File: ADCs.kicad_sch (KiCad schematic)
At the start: 25 parts, among them J10 Conn_01x03, J11 Conn_01x03, J12 Conn_01x03, J13 Conn_01x03, J14 Conn_01x03, J15 Conn_01x03, J16 Conn_01x03, J17 Conn_01x03, J2 Conn_01x03, J3 Conn_01x03, J4 Conn_01x03, J5 Conn_01x03, J6 Conn_01x03, J7 Conn_01x03, J8 Conn_01x03, J9 Conn_01x03, U13 TCA9517ADGK, U3 ADS7828, U4 ADS7828

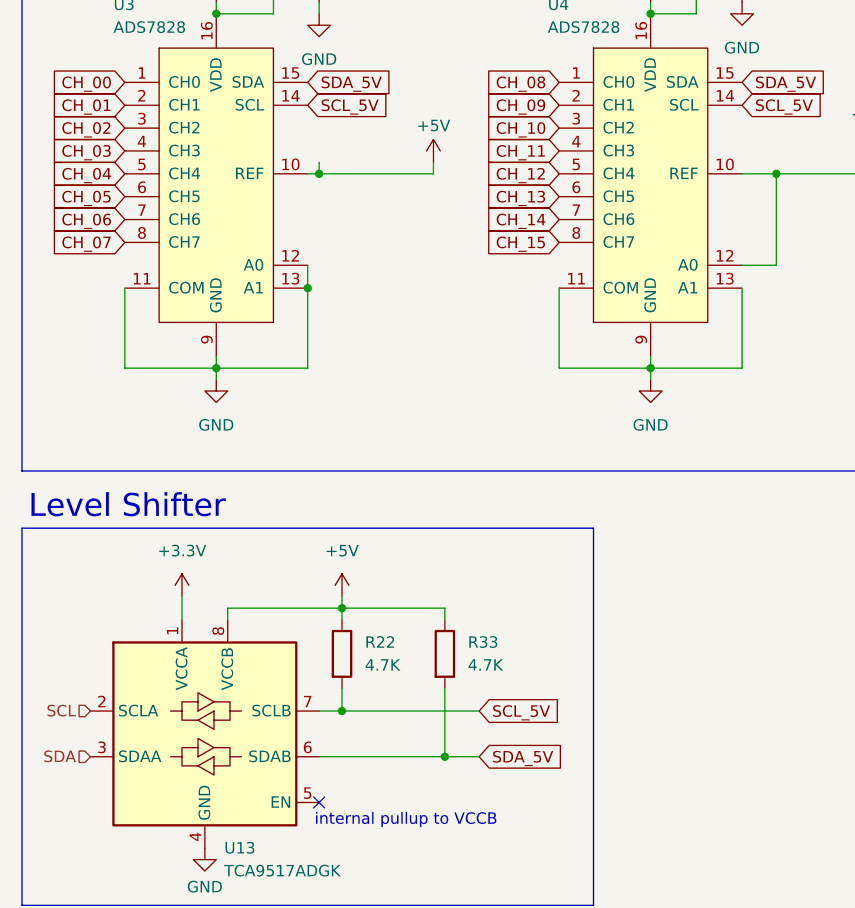
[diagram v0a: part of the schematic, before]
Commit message: First Draft of BOM
Didn't select some compoentns like diodes that I don't fully understand. Also, some components have multiple variants so we must be careful.
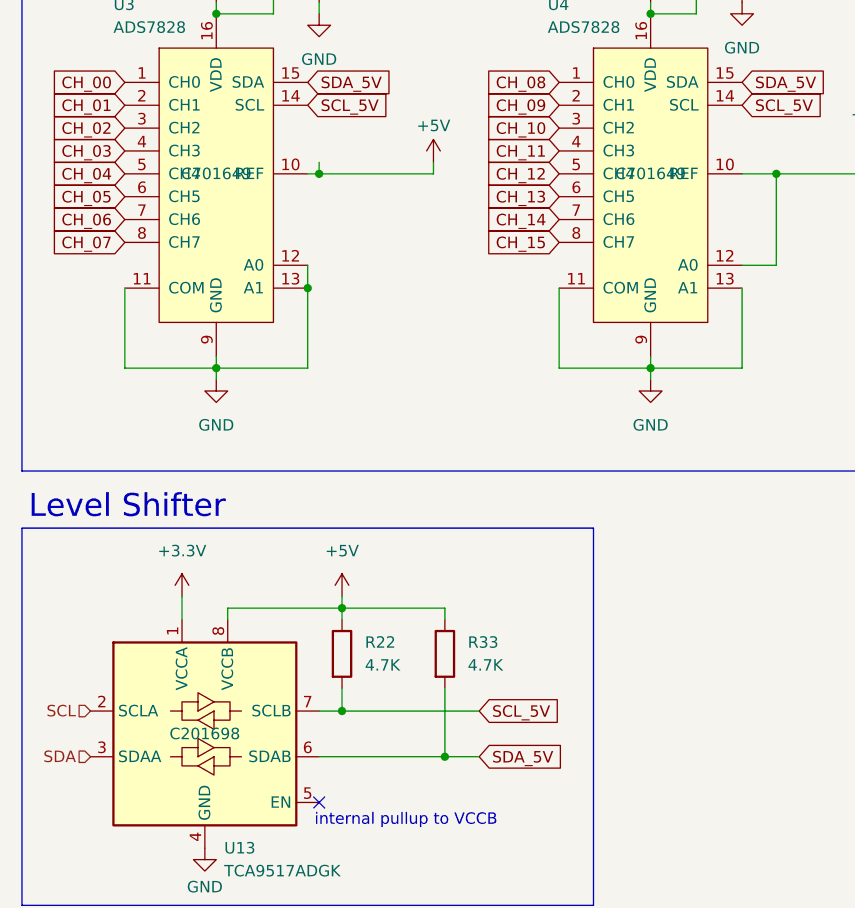
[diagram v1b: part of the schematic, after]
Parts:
- U13: JLC# (none) -> C201698
- U3, U4: JLC# (none) -> C701649
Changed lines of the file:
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@@
 			)
 		)
+		(property "JLC#" ""
+			(at 220.98 113.03 0)
+			(effects
+				(font
+					(size 1.27 1.27)
+				)
+			)
+		)
 		(pin "1"
 		)
@@
 			)
 		)
+		(property "JLC#" ""
+			(at 220.98 69.85 0)
+			(effects
+				(font
+					(size 1.27 1.27)
+				)
+			)
+		)
 		(pin "1"
 		)
@@
 			)
 		)
+		(property "JLC#" "C701649"
+			(at 124.46 93.98 0)
+			(effects
+				(font
+					(size 1.27 1.27)
+				)
+			)
+		)
 		(pin "3"
 		)
@@
 			)
 		)
+		(property "JLC#" ""
+			(at 200.66 91.44 0)
+			(effects
+				(font
+					(size 1.27 1.27)
+				)
+			)
+		)
 		(pin "1"
 		)
@@
 			)
 		)
+		(property "JLC#" "C701649"
+			(at 76.2 93.98 0)
+			(effects
+				(font
+					(size 1.27 1.27)
+				)
+			)
+		)
 		(pin "3"
 		)
@@
 			)
 		)
+		(property "JLC#" ""
+			(at 87.63 71.12 0)
+			(effects
+				(font
+					(size 1.27 1.27)
+				)
+			)
+		)
 		(pin "1"
 		)
@@
 			)
 		)
+		(property "JLC#" ""
+			(at 200.66 134.62 0)
+			(effects
+				(font
+					(size 1.27 1.27)
+				)
+			)
+		)
 		(pin "1"
 		)
@@
 			)
 		)
+		(property "JLC#" ""
+			(at 180.34 91.44 0)
+			(effects
+				(font
+					(size 1.27 1.27)
+				)
+			)
+		)
 		(pin "1"
 		)
@@
 			)
 		)
+		(property "JLC#" ""
+			(at 241.3 91.44 0)
+			(effects
+				(font
+					(size 1.27 1.27)
+				)
+			)
+		)
 		(pin "1"
 		)
@@
 			)
 		)
+		(property "JLC#" ""
+			(at 90.17 147.32 0)
+			(effects
+				(font
+					(size 1.27 1.27)
+				)
+			)
+		)
 		(pin "1"
 		)
@@
 			)
 		)
+		(property "JLC#" ""
+			(at 220.98 91.44 0)
+			(effects
+				(font
+					(size 1.27 1.27)
+				)
+			)
+		)
 		(pin "1"
 		)
@@
 			)
 		)
+		(property "JLC#" ""
+			(at 180.34 113.03 0)
+			(effects
+				(font
+					(size 1.27 1.27)
+				)
+			)
+		)
 		(pin "1"
 		)
@@
 			)
 		)
+		(property "JLC#" ""
+			(at 101.6 147.32 0)
+			(effects
+				(font
+					(size 1.27 1.27)
+				)
+			)
+		)
 		(pin "1"
 		)
@@
 			)
 		)
+		(property "JLC#" ""
+			(at 200.66 69.85 0)
+			(effects
+				(font
+					(size 1.27 1.27)
+				)
+			)
+		)
 		(pin "1"
 		)
@@
 			)
 		)
+		(property "JLC#" ""
+			(at 180.34 69.85 0)
+			(effects
+				(font
+					(size 1.27 1.27)
+				)
+			)
+		)
 		(pin "1"
 		)
@@
 			)
 		)
+		(property "JLC#" ""
+			(at 124.46 71.12 0)
+			(effects
+				(font
+					(size 1.27 1.27)
+				)
+			)
+		)
 		(pin "1"
 		)
@@
 			)
 		)
+		(property "JLC#" ""
+			(at 76.2 71.12 0)
+			(effects
+				(font
+					(size 1.27 1.27)
+				)
+			)
+		)
 		(pin "1"
 		)
@@
 			)
 		)
+		(property "JLC#" ""
+			(at 241.3 69.85 0)
+			(effects
+				(font
+					(size 1.27 1.27)
+				)
+			)
+		)
 		(pin "1"
 		)
@@
 			)
 		)
+		(property "JLC#" "C201698"
+			(at 74.93 156.21 0)
+			(effects
+				(font
+					(size 1.27 1.27)
+				)
+			)
+		)
 		(pin "7"
 		)
@@
 			)
 		)
+		(property "JLC#" ""
+			(at 134.62 71.12 0)
+			(effects
+				(font
+					(size 1.27 1.27)
+				)
+			)
+		)
 		(pin "1"
 		)
@@
 			)
 		)
+		(property "JLC#" ""
+			(at 200.66 113.03 0)
+			(effects
+				(font
+					(size 1.27 1.27)
+				)
+			)
+		)
 		(pin "1"
 		)
@@
 			)
 		)
+		(property "JLC#" ""
+			(at 241.3 113.03 0)
+			(effects
+				(font
+					(size 1.27 1.27)
+				)
+			)
+		)
 		(pin "1"
 		)
@@
 			)
 		)
+		(property "JLC#" ""
+			(at 180.34 134.62 0)
+			(effects
+				(font
+					(size 1.27 1.27)
+				)
+			)
+		)
 		(pin "1"
 		)
@@
 			)
 		)
+		(property "JLC#" ""
+			(at 220.98 134.62 0)
+			(effects
+				(font
+					(size 1.27 1.27)
+				)
+			)
+		)
 		(pin "1"
 		)
@@
 			)
 		)
+		(property "JLC#" ""
+			(at 241.3 134.62 0)
+			(effects
+				(font
+					(size 1.27 1.27)
+				)
+			)
+		)

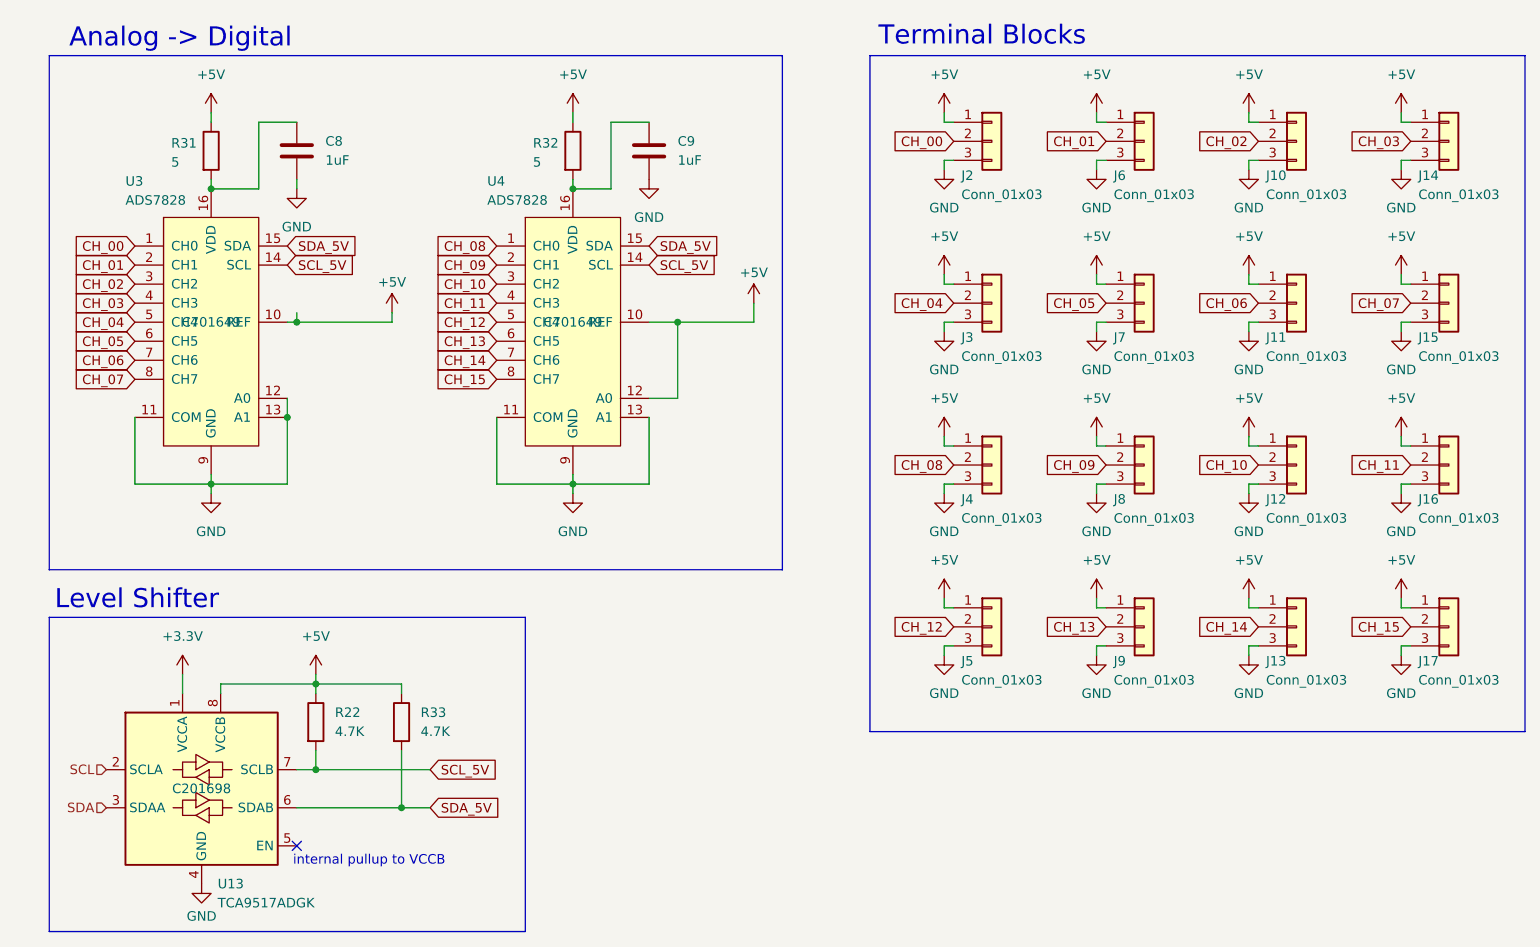
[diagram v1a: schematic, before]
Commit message: parts⚙️
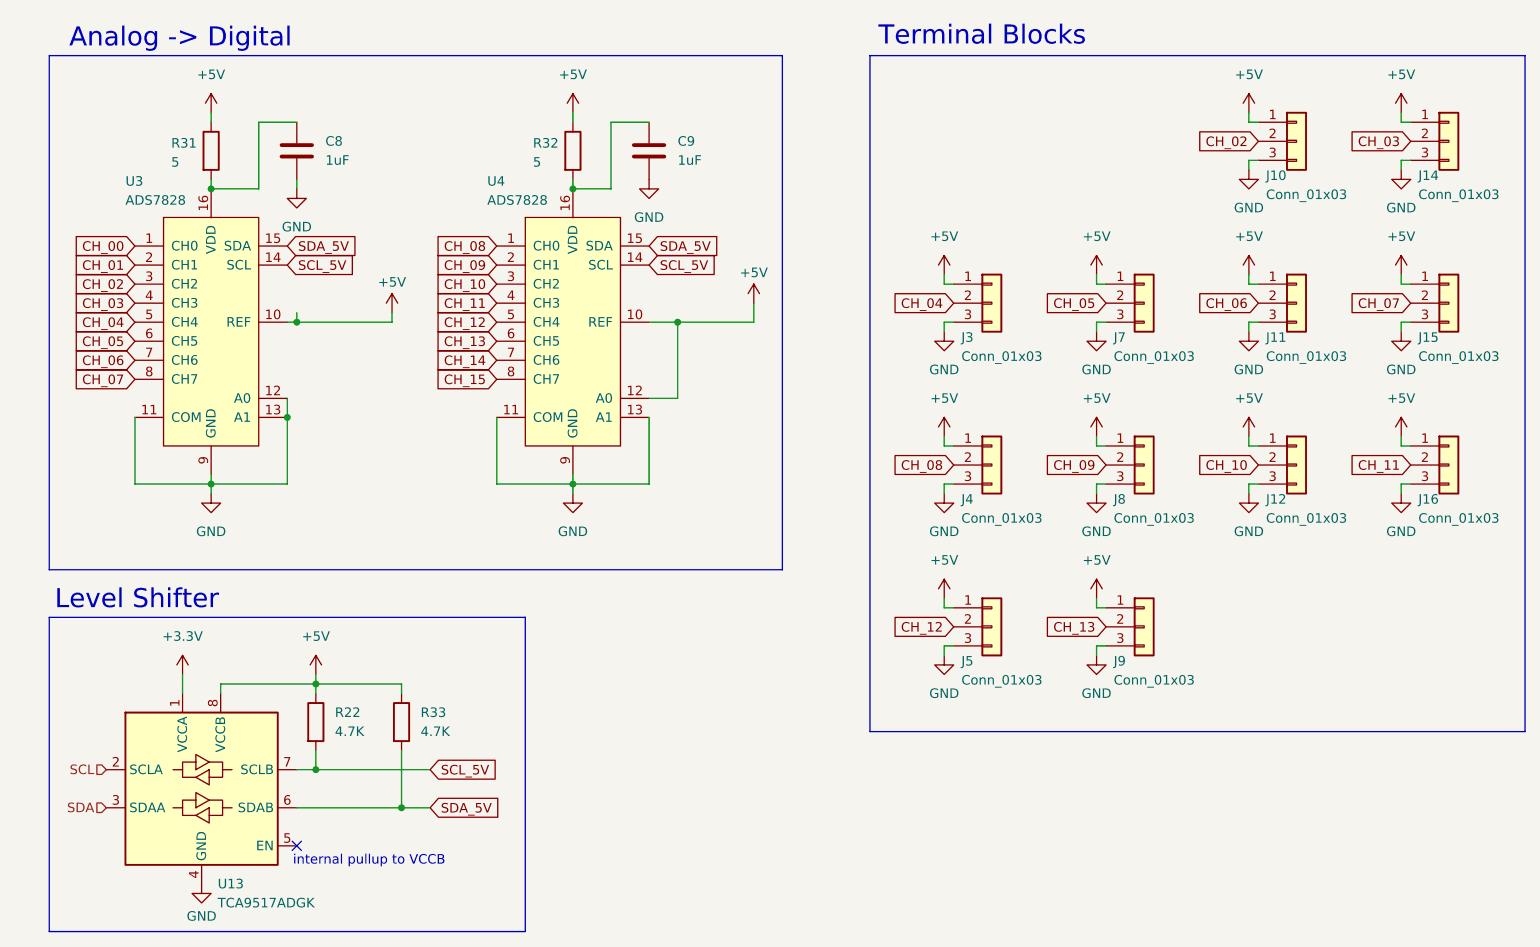
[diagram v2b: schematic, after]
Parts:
- removed J13, J17, J2, J6: Conn_01x03, TerminalBlock_Phoenix:TerminalBlock_Phoenix_MPT-0,5-3-2.54_1x03_P2.54mm_Horizontal, symbol Connector_Generic:Conn_01x03
- J10, J11, J12, J14, J15, J16, J3, J4, J5, J7, J8, J9: JLC# (none) -> C918121
- U13: JLC# C201698 -> C201698
- U3, U4: JLC# C701649 -> C701649

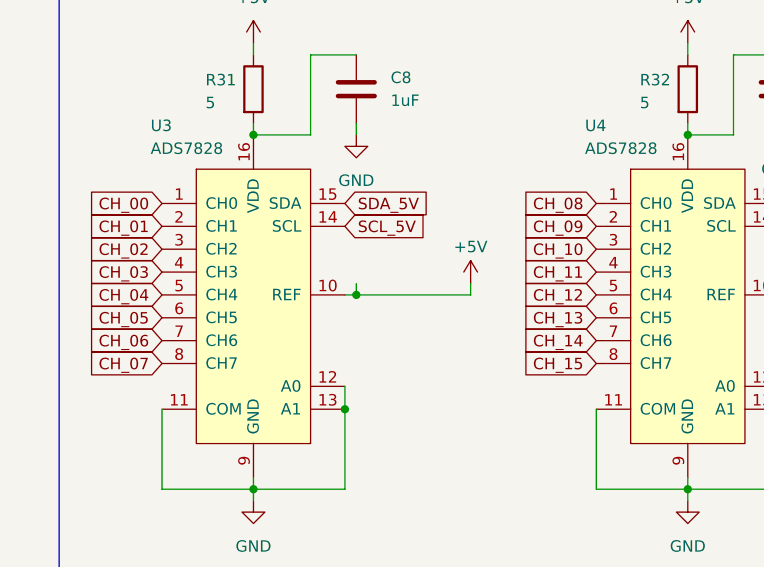
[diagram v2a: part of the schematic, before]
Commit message: touchups 💅
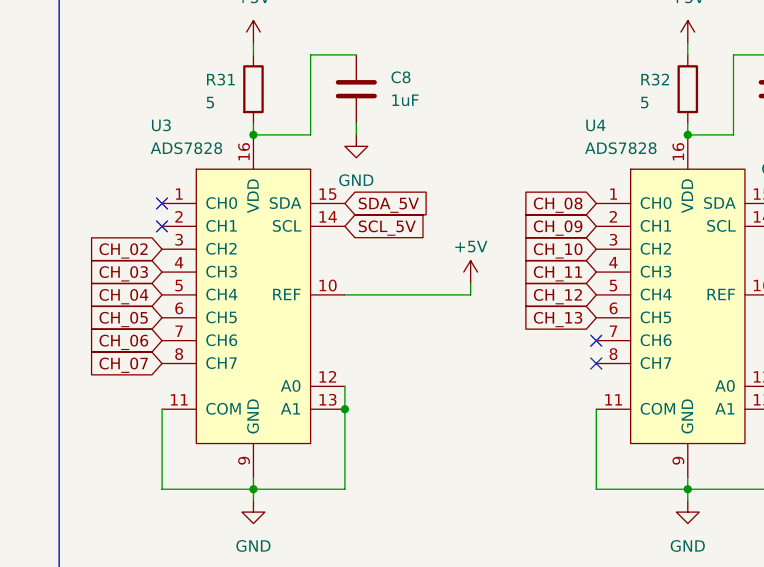
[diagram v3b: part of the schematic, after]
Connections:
- net CH_00: no longer names the net of U3.1 (CH0)
- net CH_01: no longer names the net of U3.2 (CH1)
- net CH_14: no longer names the net of U4.7 (CH6)
- net CH_15: no longer names the net of U4.8 (CH7)
- no-connect marks 1 -> 5
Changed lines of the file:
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@@
-	)
-	(junction
-		(at 87.63 93.98)
-		(diameter 0)
-		(color 0 0 0 0)
 	)
 	(junction
@@
 	)
 	(no_connect
+		(at 114.3 99.06)
+	)
+	(no_connect
+		(at 66.04 86.36)
+	)
+	(no_connect
+		(at 66.04 83.82)
+	)
+	(no_connect
 		(at 87.63 163.83)
 	)
+	(no_connect
+		(at 114.3 101.6)
+	)
 	(wire
 		(pts
@@
 	(wire
 		(pts
-			(xy 87.63 92.71) (xy 87.63 93.98)
-		)
-		(stroke
-			(width 0)
-			(type default)
-		)
-	)
-	(wire
-		(pts
 			(xy 72.39 140.97) (xy 72.39 143.51)
 		)
@@
 	(wire
 		(pts
-			(xy 87.63 93.98) (xy 100.33 93.98)
+			(xy 86.36 93.98) (xy 100.33 93.98)
 		)
 		(stroke
@@
 	(wire
 		(pts
-			(xy 86.36 93.98) (xy 87.63 93.98)
-		)
-		(stroke
-			(width 0)
-			(type default)
-		)
-	)
-	(wire
-		(pts
 			(xy 134.62 67.31) (xy 129.54 67.31)
 		)
@@
 		)
 	)
-	(global_label "CH_00"
-		(shape input)
-		(at 66.04 83.82 180)
-		(fields_autoplaced yes)
-		(effects
-			(font
-				(size 1.27 1.27)
-			)
-			(justify right)
-		)
-		(property "Intersheetrefs" "${INTERSHEET_REFS}"
-			(at 57.0677 83.82 0)
-			(effects
-				(font
-					(size 1.27 1.27)
-				)
-				(justify right)
-				(hide yes)
-			)
-		)
-	)
 	(global_label "CH_12"
 		(shape input)
@@
 		)
 	)
-	(global_label "CH_01"
-		(shape input)
-		(at 66.04 86.36 180)
-		(fields_autoplaced yes)
-		(effects
-			(font
-				(size 1.27 1.27)
-			)
-			(justify right)
-		)
-		(property "Intersheetrefs" "${INTERSHEET_REFS}"
-			(at 57.0677 86.36 0)
-			(effects
-				(font
-					(size 1.27 1.27)
-				)
-				(justify right)
-				(hide yes)
-			)
-		)
-	)
-	(global_label "CH_15"
-		(shape input)
-		(at 114.3 101.6 180)
-		(fields_autoplaced yes)
-		(effects
-			(font
-				(size 1.27 1.27)
-			)
-			(justify right)
-		)
-		(property "Intersheetrefs" "${INTERSHEET_REFS}"
-			(at 105.3277 101.6 0)
-			(effects
-				(font
-					(size 1.27 1.27)
-				)
-				(justify right)
-				(hide yes)
-			)
-		)
-	)
 	(global_label "CH_10"
 		(shape input)
@@
 			(effects
 				(font
-					(size 1.27 1.27)
-				)
-				(justify right)
-				(hide yes)
-			)
-		)
-	)
-	(global_label "CH_14"
-		(shape input)
-		(at 114.3 99.06 180)
-		(fields_autoplaced yes)
-		(effects
-			(font
-				(size 1.27 1.27)
-			)
-			(justify right)
-		)
-		(property "Intersheetrefs" "${INTERSHEET_REFS}"
-			(at 105.3277 99.06 0)
-			(effects
-				(font
